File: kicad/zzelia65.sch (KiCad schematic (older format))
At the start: 138 parts

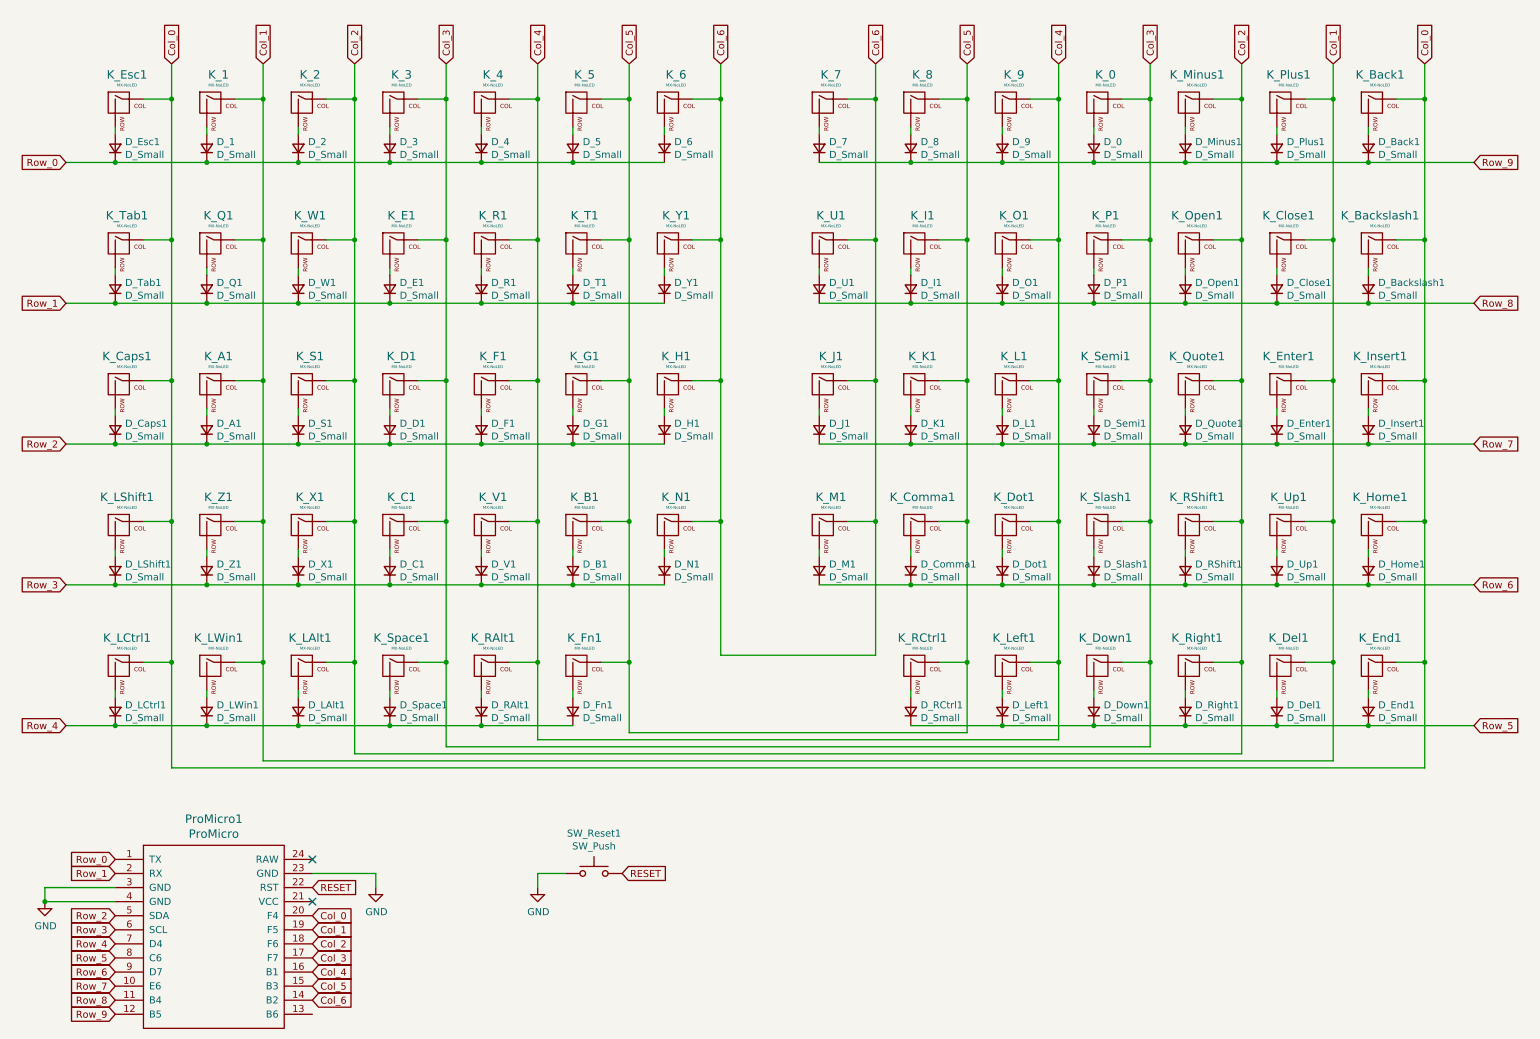
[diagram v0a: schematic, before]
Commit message: 18-pin
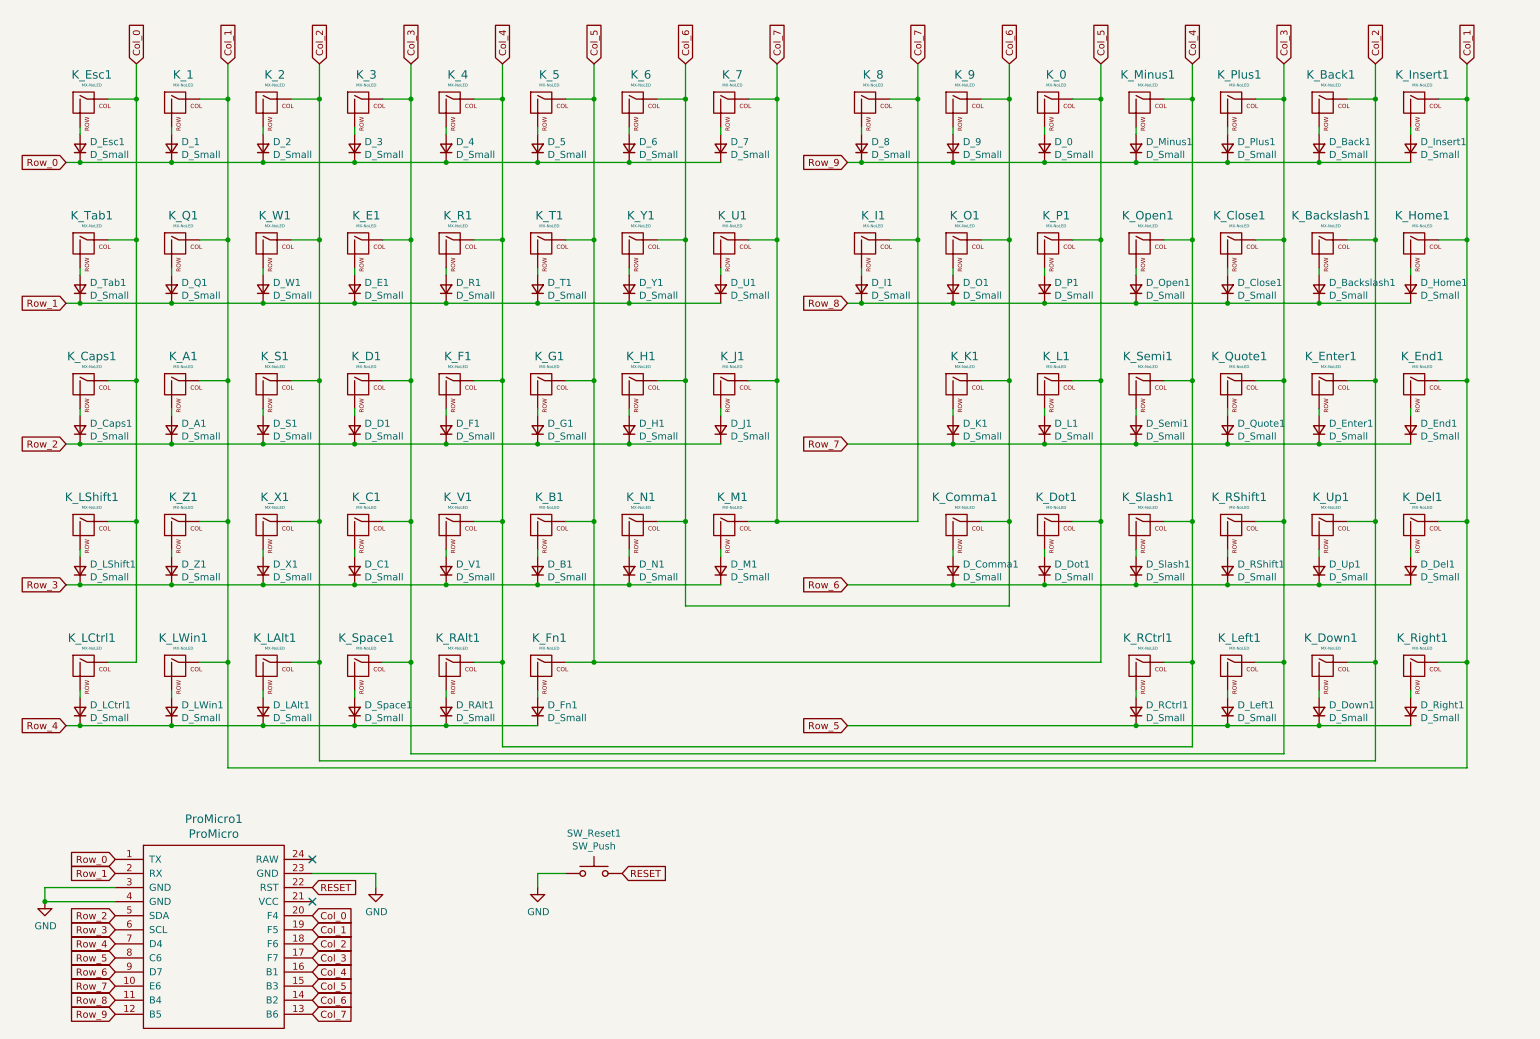
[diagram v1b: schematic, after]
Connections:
- net Col_0: no longer K_Back1.1 (COL), K_Backslash1.1 (COL), K_End1.1 (COL), K_Home1.1 (COL), K_Insert1.1 (COL)
- net Col_1: now also K_End1.1 (COL), K_Home1.1 (COL), K_Insert1.1 (COL), K_Right1.1 (COL); no longer K_Close1.1 (COL), K_Enter1.1 (COL), K_Plus1.1 (COL), K_Up1.1 (COL)
- net Col_2: now also K_Back1.1 (COL), K_Backslash1.1 (COL), K_Down1.1 (COL), K_Enter1.1 (COL), K_Up1.1 (COL); no longer K_Minus1.1 (COL), K_Open1.1 (COL), K_Quote1.1 (COL), K_RShift1.1 (COL), K_Right1.1 (COL)
- net Col_3: now also K_Close1.1 (COL), K_Left1.1 (COL), K_Plus1.1 (COL), K_Quote1.1 (COL), K_RShift1.1 (COL); no longer K_0.1 (COL), K_Down1.1 (COL), K_P1.1 (COL), K_Semi1.1 (COL), K_Slash1.1 (COL)
- net Col_4: now also K_Minus1.1 (COL), K_Open1.1 (COL), K_RCtrl1.1 (COL), K_Semi1.1 (COL), K_Slash1.1 (COL); no longer K_9.1 (COL), K_Dot1.1 (COL), K_L1.1 (COL), K_Left1.1 (COL), K_O1.1 (COL)
- net Col_5: now also K_0.1 (COL), K_Dot1.1 (COL), K_L1.1 (COL), K_P1.1 (COL); no longer K_8.1 (COL), K_Comma1.1 (COL), K_I1.1 (COL), K_K1.1 (COL), K_RCtrl1.1 (COL)
- net Col_6: now also K_9.1 (COL), K_Comma1.1 (COL), K_K1.1 (COL), K_O1.1 (COL); no longer K_7.1 (COL), K_J1.1 (COL), K_M1.1 (COL), K_U1.1 (COL)
- net Row_0: now also D_7.1 (K)
- net Row_1: now also D_U1.1 (K)
- net Row_2: now also D_J1.1 (K)
- net Row_3: now also D_M1.1 (K)
- net Row_5: no longer D_Del1.1 (K), D_End1.1 (K)
- net Row_6: now also D_Del1.1 (K); no longer D_Home1.1 (K), D_M1.1 (K)
- net Row_7: now also D_End1.1 (K); no longer D_Insert1.1 (K), D_J1.1 (K)
- net Row_8: now also D_Home1.1 (K); no longer D_U1.1 (K)
- net Row_9: now also D_Insert1.1 (K); no longer D_7.1 (K)
- net Col_7: now reaches ProMicro1.13 (B6)
- net Col_7: now also K_7.1 (COL), K_8.1 (COL), K_I1.1 (COL), K_J1.1 (COL), K_M1.1 (COL), K_U1.1 (COL)
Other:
- moved on the sheet: D_0, D_1, D_2, D_3, D_4, D_5, D_6, D_7, D_8, D_9, D_A1, D_B1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

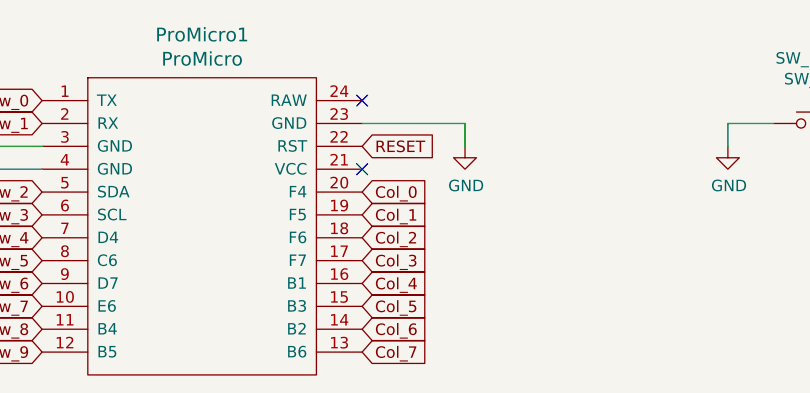
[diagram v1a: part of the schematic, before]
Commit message: routing
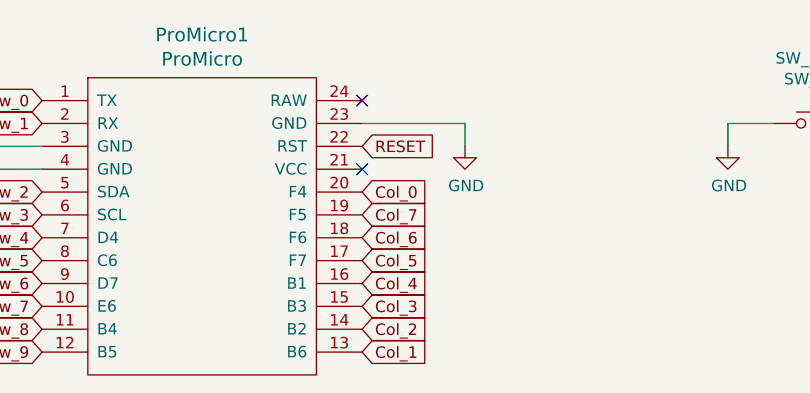
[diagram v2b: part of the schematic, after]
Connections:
- net Col_1: now also ProMicro1.13 (B6); no longer ProMicro1.19 (F5)
- net Col_2: now also ProMicro1.14 (B2); no longer ProMicro1.18 (F6)
- net Col_3: now also ProMicro1.15 (B3); no longer ProMicro1.17 (F7)
- net Col_5: now also ProMicro1.17 (F7); no longer ProMicro1.15 (B3)
- net Col_6: now also ProMicro1.18 (F6); no longer ProMicro1.14 (B2)
- net Col_7: now also ProMicro1.19 (F5); no longer ProMicro1.13 (B6)
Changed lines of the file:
@@
 Text GLabel 2500 6850 2    50   Input ~ 0
 Col_0
-Text GLabel 2500 6950 2    50   Input ~ 0
+Text GLabel 2500 7550 2    50   Input ~ 0
 Col_1
-Text GLabel 2500 7050 2    50   Input ~ 0
+Text GLabel 2500 7450 2    50   Input ~ 0
 Col_2
-Text GLabel 2500 7150 2    50   Input ~ 0
+Text GLabel 2500 7350 2    50   Input ~ 0
 Col_3
 Text GLabel 2500 7250 2    50   Input ~ 0
 Col_4
-Text GLabel 2500 7350 2    50   Input ~ 0
+Text GLabel 2500 7150 2    50   Input ~ 0
 Col_5
-Text GLabel 2500 7450 2    50   Input ~ 0
+Text GLabel 2500 7050 2    50   Input ~ 0
 Col_6
 Wire Wire Line
@@
 	10700 5050 10700 5800
 Connection ~ 1900 5050
-Text GLabel 2500 7550 2    50   Input ~ 0
+Text GLabel 2500 6950 2    50   Input ~ 0
 Col_7
 $EndSCHEMATC
